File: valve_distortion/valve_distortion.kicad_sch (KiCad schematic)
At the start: 30 parts, among them J1 INPUT, J2 OUTPUT, J3 Barrel_Jack, SW1 SW_DPDT_x2, U1 12AX7, U2 TL074

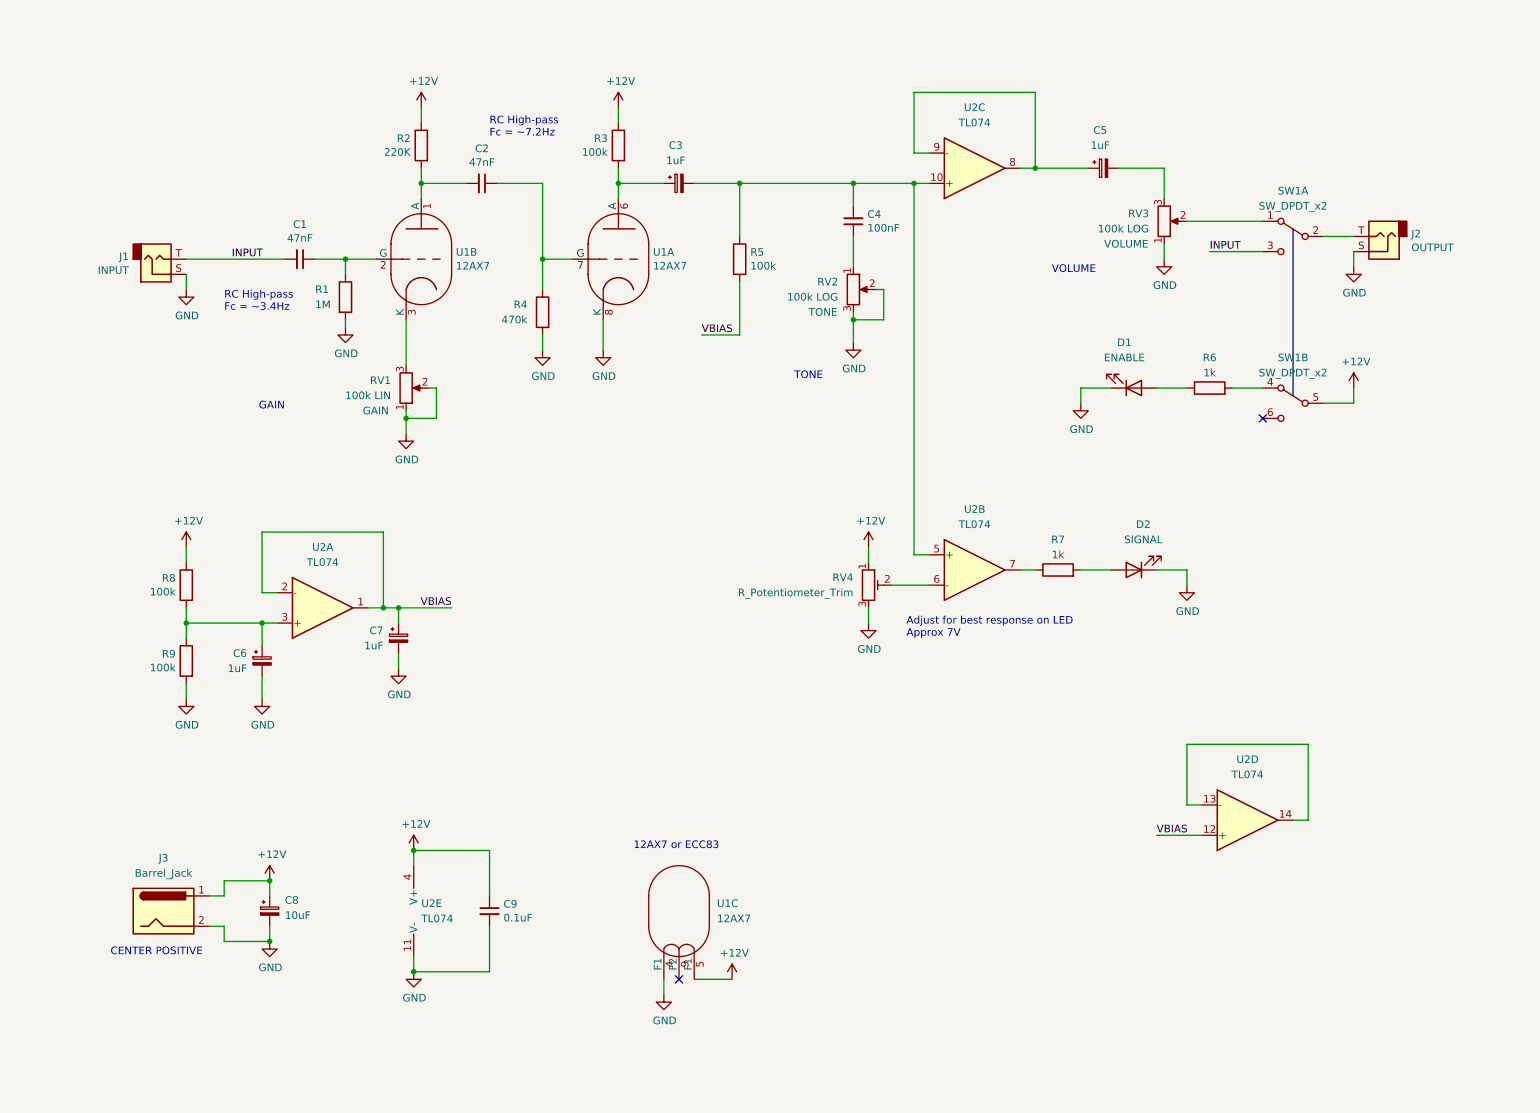
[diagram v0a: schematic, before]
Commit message: Finish layout
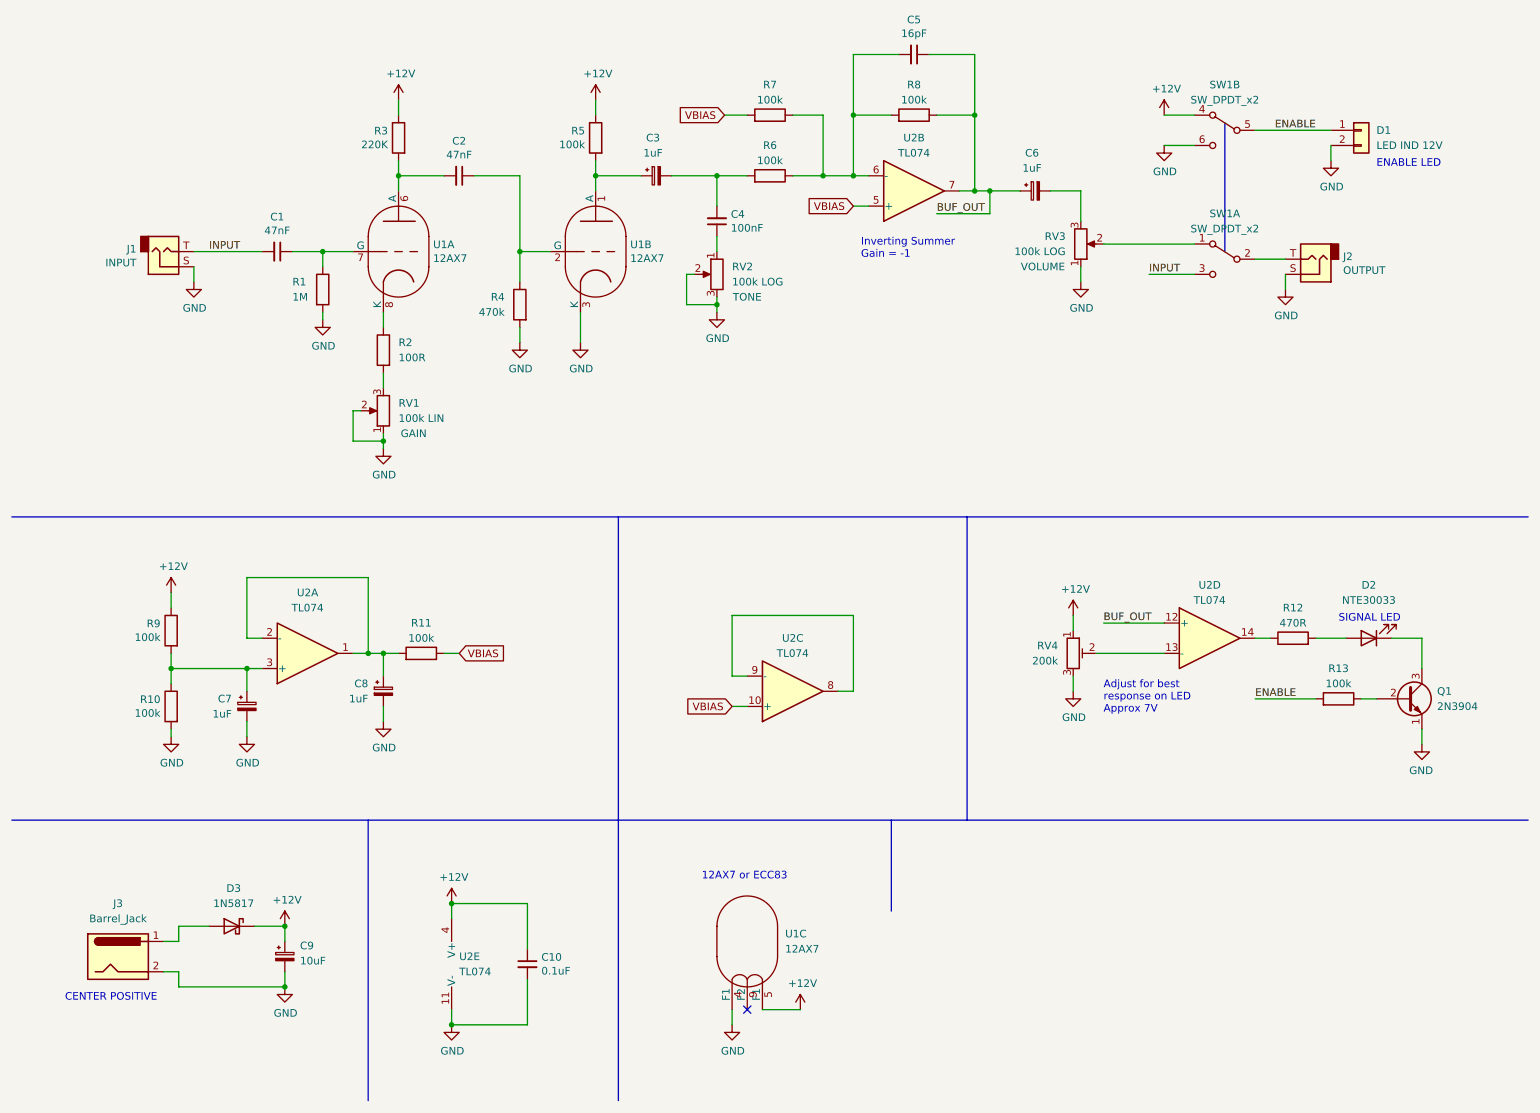
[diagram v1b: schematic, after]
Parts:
- removed D1: ENABLE, Connector_PinHeader_2.54mm:PinHeader_1x02_P2.54mm_Vertical, symbol Device:LED
- removed R5: 100k, Resistor_THT:R_Axial_DIN0207_L6.3mm_D2.5mm_P10.16mm_Horizontal, symbol Device:R
- added C5: 16pF, Capacitor_THT:C_Disc_D3.0mm_W1.6mm_P2.50mm, symbol Device:C_Small
- added D1: LED IND 12V, Connector_PinHeader_2.54mm:PinHeader_1x02_P2.54mm_Vertical, symbol Connector_Generic:Conn_01x02
- added D3: 1N5817, Diode_THT:D_DO-41_SOD81_P10.16mm_Horizontal, symbol Diode:1N5817
- added Q1: 2N3904, Package_TO_SOT_THT:TO-92_Inline, symbol Transistor_BJT:2N3904
- added R11, R13, R7, R8: 100k, Resistor_THT:R_Axial_DIN0207_L6.3mm_D2.5mm_P10.16mm_Horizontal, symbol Device:R
- added R2: 100R, Resistor_THT:R_Axial_DIN0207_L6.3mm_D2.5mm_P10.16mm_Horizontal, symbol Device:R
- D2: value SIGNAL -> NTE30033
- J1, J2: footprint Connector_Molex:Molex_KK-254_AE-6410-02A_1x02_P2.54mm_Vertical -> Connector_PinHeader_2.54mm:PinHeader_1x02_P2.54mm_Vertical
- R12: renamed from R7; value 1k -> 470R
- R6: value 1k -> 100k
- RV4: value R_Potentiometer_Trim -> 200k; footprint Potentiometer_THT:Potentiometer_Bourns_3266Y_Vertical -> valve_distortion:Trimmer
- renumbered C9 to C10, C5 to C6, C6 to C7, C7 to C8, C8 to C9, R9 to R10, R2 to R3, R3 to R5, R8 to R9
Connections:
- net +12V: now also SW1.4 (A), D3.1 (K); no longer J3.1, SW1.5 (B)
- net GND: now also SW1.6 (C), U1.3 (K), D1.2 (Pin_2), Q1.1 (E); no longer D2.1 (K), U1.8 (K)
- net VBIAS: now also U2.10 (+), U2.5 (+), R11.1, R7.2; no longer C8.1, U2.1, U2.12 (+), U2.2 (-)
- net at C3.1, R5.2: now also U1.1 (A); no longer U1.6 (A)
- net at C2.1, R4.1: now also U1.2 (G); no longer U1.7 (G)
- net at C2.2, R3.2: now also U1.6 (A); no longer U1.1 (A)
- net at C1.1, R1.1: now also U1.7 (G); no longer U1.2 (G)
- net at RV1.3: now also R2.2; no longer U1.3 (K)
- net at C3.2, C4.2: now also R6.2; no longer U2.10 (+), U2.5 (+)
- net at U2.6 (-): now also R6.1, C5.2, R7.1, R8.2; no longer RV4.2
- net at R12.1: now also U2.14; no longer U2.7
- net at U2.8, U2.9 (-): no longer C6.1
- net at U2.13 (-): now also RV4.2; no longer U2.14
- new net: R2.1, U1.8 (K)
- new net: C8.1, R11.2, U2.1, U2.2 (-)
- new net: Q1.2 (B), R13.1
- new net: D2.1 (K), Q1.3 (C)
- new net: D3.2 (A), J3.1
- new net BUF_OUT: C5.1, C6.1, R8.1, U2.12 (+), U2.7
- new net ENABLE: D1.1 (Pin_1), R13.2, SW1.5 (B)
- no-connect marks 2 -> 1
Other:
- note added: "ENABLE LED"
- note added: "Inverting Summer Gain = -1"
- note added: "SIGNAL LED"
- note removed: "GAIN"
- note removed: "RC High-pass Fc = ~3.4Hz"
- note removed: "RC High-pass Fc = ~7.2Hz"
- note removed: "TONE"
- note removed: "VOLUME"
- moved on the sheet: C1, C10, C2, C3, C6, C7, C8, C9, D2, J1, J2, J3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
